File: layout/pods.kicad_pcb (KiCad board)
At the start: 2 copper layers, 50 x 80 mm, 29 parts, among them J1 BATTERY, U1 STM32F103RCT6, U2 nRF24L01+, U4 ADP1710AUJZ, U5 SWD, U6 TP4056, U7 SH1106

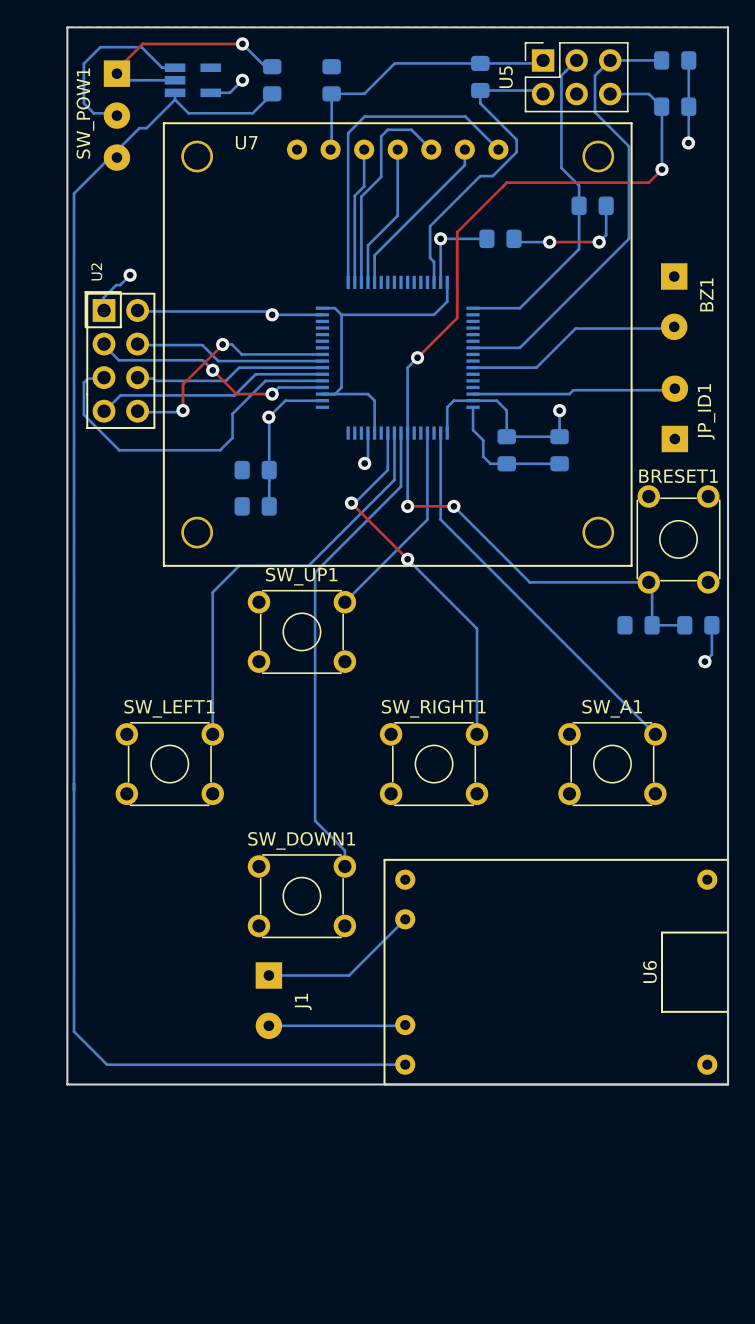
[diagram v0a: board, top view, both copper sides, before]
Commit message: Updated schematic/pcb
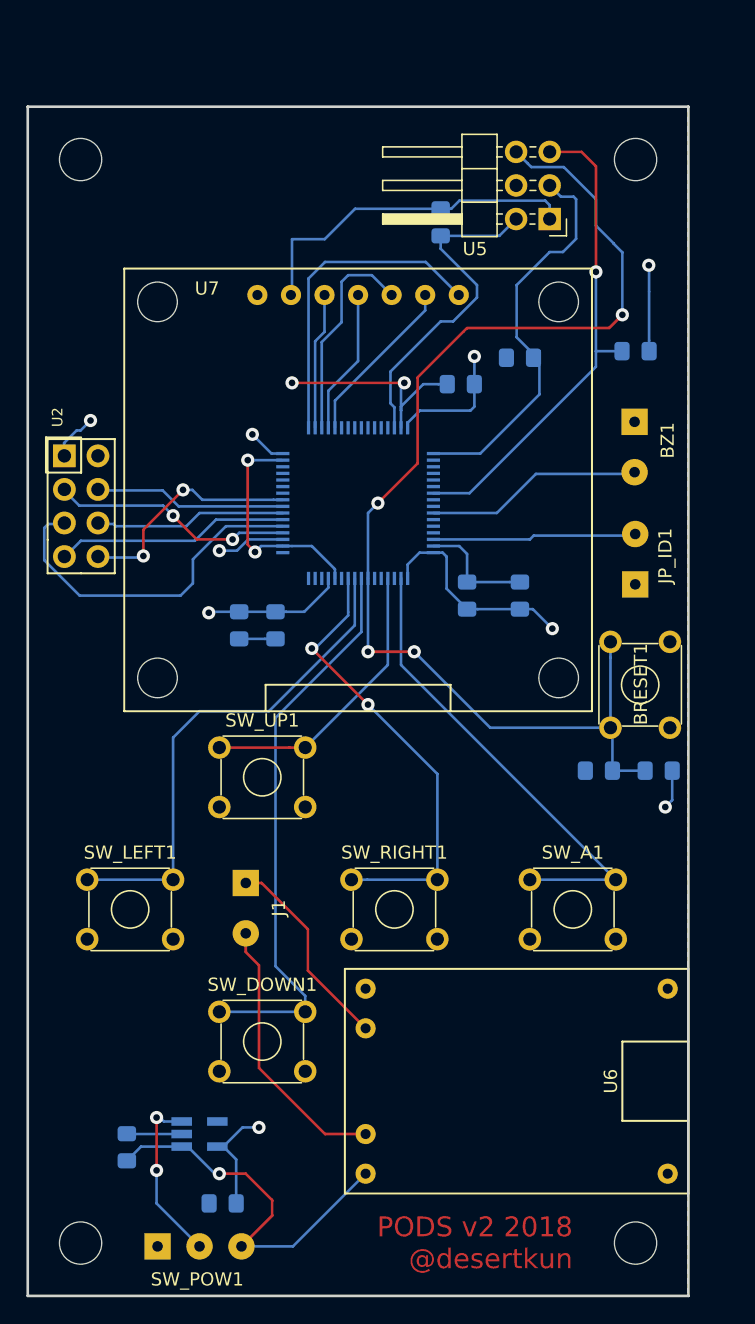
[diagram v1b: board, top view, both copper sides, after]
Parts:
- removed R4: 10K, Resistor_SMD:R_0805_2012Metric_Pad1.15x1.40mm_HandSolder
- added REF**: MountingHole_3.2mm_M3, MountingHole:MountingHole_3.2mm_M3, F.Cu at (116.7, 54.5)
- added REF**: MountingHole_3.2mm_M3, MountingHole:MountingHole_3.2mm_M3, F.Cu at (74.7, 54.5)
- added REF**: MountingHole_3.2mm_M3, MountingHole:MountingHole_3.2mm_M3, F.Cu at (74.7, 136.5)
- added REF**: MountingHole_3.2mm_M3, MountingHole:MountingHole_3.2mm_M3, F.Cu at (116.7, 136.5)
- BRESET1, SW_A1, SW_DOWN1, SW_LEFT1, SW_RIGHT1, SW_UP1: footprint Button_Switch_THT:SW_TH_Tactile_Omron_B3F-10xx -> switches:SW_TH_Tactile_Omron_Fixed
- U5: footprint Connector_PinSocket_2.54mm:PinSocket_2x03_P2.54mm_Vertical -> Connector_PinHeader_2.54mm:PinHeader_2x03_P2.54mm_Horizontal
- moved SW_POW1 88.8 mm to (80.5, 136.7), turned to 0 degrees
- moved C2 85.4 mm to (85.4, 133.5), turned to 180 degrees
- moved C1 81.5 mm to (78.2, 129.2)
- moved U4 79.8 mm to (83.7, 128.2)
- moved R5 22.2 mm to (116.7, 69.0)
- moved R2 12.7 mm to (107.9, 69.5), turned to 0 degrees
- moved U5 12.0 mm to (110.2, 59.0), turned to 180 degrees
- moved C7 11.8 mm to (86.7, 89.7), turned to 270 degrees
- moved BZ1 11.4 mm to (116.6, 74.3)
- moved C3 11.4 mm to (107.9, 87.5), turned to 90 degrees
- moved C4 11.4 mm to (103.9, 87.5), turned to 90 degrees
- moved C8 11.4 mm to (113.9, 100.7)
- moved JP_ID1 11.4 mm to (116.6, 86.6)
- moved R1 11.4 mm to (101.9, 59.2)
- moved R3 11.4 mm to (118.4, 100.7)
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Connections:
- U1 pad 18: +3V3 -> GND
- U1 pad 19: GND -> +3V3
- U1 pad 31: +3V3 -> GND
- U1 pad 32: GND -> +3V3
- U1 pad 47: +3V3 -> GND
- U1 pad 48: GND -> +3V3
- U1 pad 63: +3V3 -> GND
- U1 pad 64: GND -> +3V3
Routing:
- net +4V: track 109.5 -> 29.3 mm, vias 0 -> 1
- net RESET: track 75.3 -> 89.8 mm
- net GND: track 66.7 -> 53.6 mm, vias 4 -> 5
- net +BATT: track 10.3 -> 20.7 mm
- net BUTTON_UP: track 15.4 -> 21.9 mm
- net BUTTON_RIGHT: track 28.0 -> 34.5 mm
- net BUTTON_LEFT: track 31.6 -> 38.1 mm
- net BUTTON_DOWN: track 36.4 -> 42.9 mm
- net BUTTON_A: track 29.5 -> 36.0 mm
- net SWCLK: track 25.2 -> 30.6 mm
- net +3V3: track 82.9 -> 88.2 mm
- net -BATT: track 12.1 -> 15.5 mm
- net SWO: track 34.2 -> 37.4 mm, vias 0 -> 1
- net SWDIO: track 23.9 -> 25.3 mm
- net Net-(SW_POW1-Pad2): track 14.1 -> 13.1 mm, vias 0 -> 2
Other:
- board size 50 x 80 mm -> 50 x 90 mm
- board text added: "PODS v2 2018 @desertkun"
